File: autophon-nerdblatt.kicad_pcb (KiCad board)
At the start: 2 copper layers, 265 x 50.6 mm, 116 parts, among them J1 Conn_01x06_Female, J101 board-edge-connector, J2 Conn_02x06_Odd_Even, Q300 BSS84, Q301 BSS84, Q302 BSS84, Q303 BSS84, Q304 BSS84, Q305 BSS84, SW1 SW_Push, SW2 SW_Push, U1 EA_W096016-XALW, U101 LM1117-3.3, U102 LM2594M-5.0, U201 SN74LV1T34, U202 SN74LV1T34, U203 74AHCT595, U204 SN74LV1T34, U205 74AHCT595, U206 ESP32-WROOM-32, U207 74AHCT595, U300 L298HN, U301 L298HN, U302 L298HN

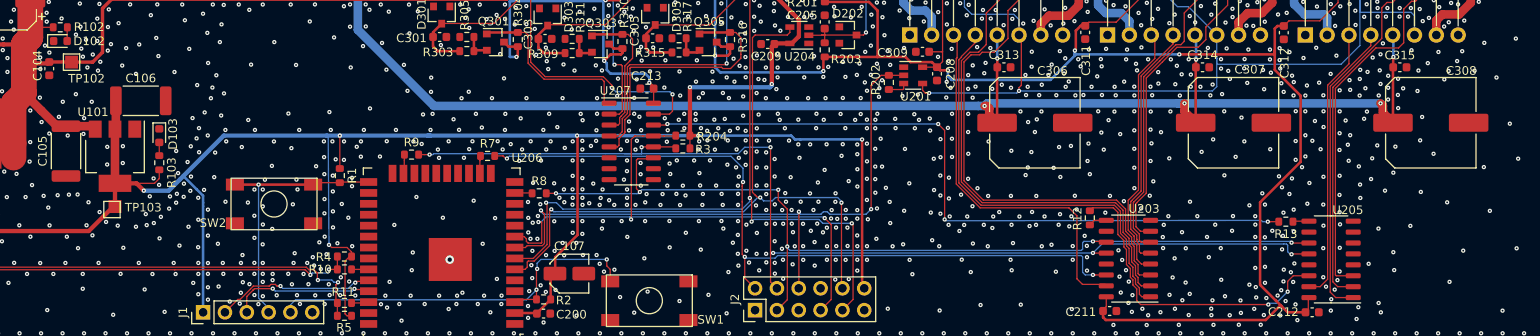
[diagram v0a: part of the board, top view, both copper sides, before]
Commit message: BOM
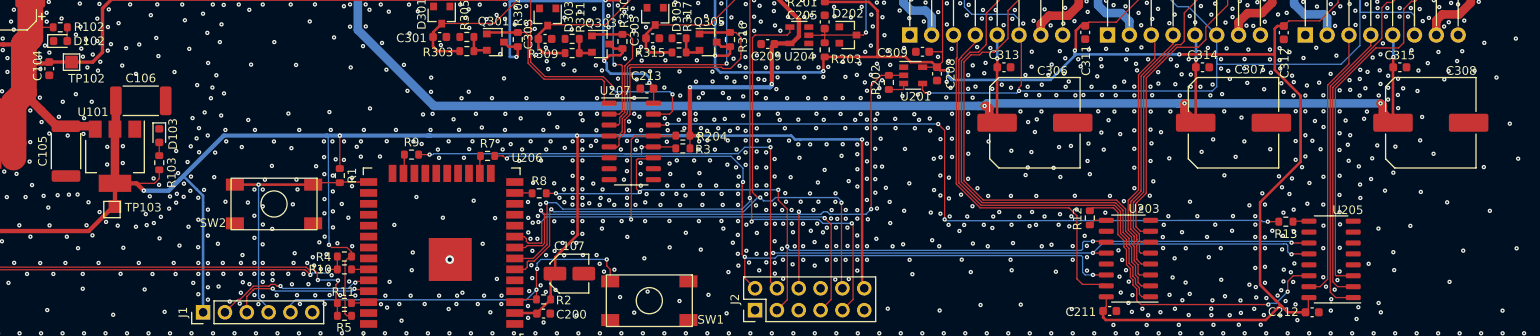
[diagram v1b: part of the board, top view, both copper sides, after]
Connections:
- J101 pad 12A: no_connect_112 -> no_connect_113
- J101 pad 13A: no_connect_113 -> no_connect_114
- J101 pad 14A: no_connect_114 -> no_connect_115
- J101 pad 15A: no_connect_115 -> no_connect_116
- J101 pad 15B: no_connect_116 -> no_connect_117
- J101 pad 16A: no_connect_117 -> no_connect_118
- J101 pad 16B: no_connect_118 -> no_connect_119
- J101 pad 17A: no_connect_119 -> no_connect_120
- J101 pad 18A: no_connect_120 -> no_connect_121
- J101 pad 19A: no_connect_121 -> no_connect_122
- J101 pad 1A: no_connect_122 -> no_connect_123
- J101 pad 1B: no_connect_123 -> no_connect_124
- J101 pad 20A: no_connect_124 -> no_connect_125
- J101 pad 21A: no_connect_125 -> no_connect_126
- J101 pad 21B: no_connect_126 -> no_connect_127
- J101 pad 22A: no_connect_127 -> no_connect_128
- J101 pad 22B: no_connect_128 -> no_connect_129
- J101 pad 23B: no_connect_129 -> no_connect_130
- J101 pad 24B: no_connect_130 -> no_connect_131
- J101 pad 25B: no_connect_131 -> no_connect_132
- J101 pad 26A: no_connect_132 -> no_connect_133
- J101 pad 26B: no_connect_133 -> no_connect_134
- J101 pad 27B: no_connect_134 -> no_connect_135
- J101 pad 28B: no_connect_135 -> no_connect_136
- J101 pad 29B: no_connect_136 -> no_connect_137
- J101 pad 2A: no_connect_137 -> no_connect_138
- J101 pad 2B: no_connect_138 -> no_connect_139
- J101 pad 30A: no_connect_139 -> no_connect_140
- J101 pad 30B: no_connect_140 -> no_connect_141
- J101 pad 31B: no_connect_141 -> no_connect_142
- J101 pad 32B: no_connect_142 -> no_connect_143
- J101 pad 33B: no_connect_143 -> no_connect_144
- J101 pad 34A: no_connect_144 -> no_connect_145
- J101 pad 36B: no_connect_145 -> no_connect_146
- J101 pad 38A: no_connect_146 -> no_connect_147
- J101 pad 38B: no_connect_147 -> no_connect_148
- J101 pad 39A: no_connect_148 -> no_connect_149
- J101 pad 3A: no_connect_149 -> no_connect_150
- J101 pad 3B: no_connect_150 -> no_connect_151
- J101 pad 40A: no_connect_151 -> no_connect_152
- J101 pad 40B: no_connect_152 -> no_connect_153
- J101 pad 41A: no_connect_153 -> no_connect_154
- J101 pad 41B: no_connect_154 -> no_connect_155
- J101 pad 42A: no_connect_155 -> no_connect_156
- J101 pad 42B: no_connect_156 -> no_connect_157
- J101 pad 43A: no_connect_157 -> no_connect_158
- J101 pad 43B: no_connect_158 -> no_connect_159
- J101 pad 44A: no_connect_159 -> no_connect_160
- J101 pad 44B: no_connect_160 -> no_connect_161
- J101 pad 4A: no_connect_161 -> no_connect_162
- J101 pad 4B: no_connect_162 -> no_connect_163
- J101 pad 5A: no_connect_163 -> no_connect_164
- J101 pad 5B: no_connect_164 -> no_connect_165
- J101 pad 6B: no_connect_165 -> no_connect_166
- J101 pad 7A: no_connect_166 -> no_connect_167
- J101 pad 7B: no_connect_167 -> no_connect_168
- J101 pad 8B: no_connect_168 -> no_connect_169
- J101 pad 9A: no_connect_169 -> no_connect_170
- U203 pad 10: ABCDEF_HALL_GND -> Net-(U203-Pad10)
- U206 pad 17: no_connect_170 -> no_connect_171
- U206 pad 18: no_connect_171 -> no_connect_172
- U206 pad 19: no_connect_172 -> no_connect_173
- U206 pad 20: no_connect_173 -> no_connect_174
- U206 pad 21: no_connect_174 -> no_connect_175
- U206 pad 22: no_connect_175 -> no_connect_176
- U206 pad 24: no_connect_176 -> no_connect_177
- U206 pad 4: no_connect_177 -> no_connect_178
- U206 pad 5: no_connect_178 -> no_connect_179
